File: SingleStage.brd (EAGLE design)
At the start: 47.9 x 35.5 mm, 29 parts, among them T1 2N5089

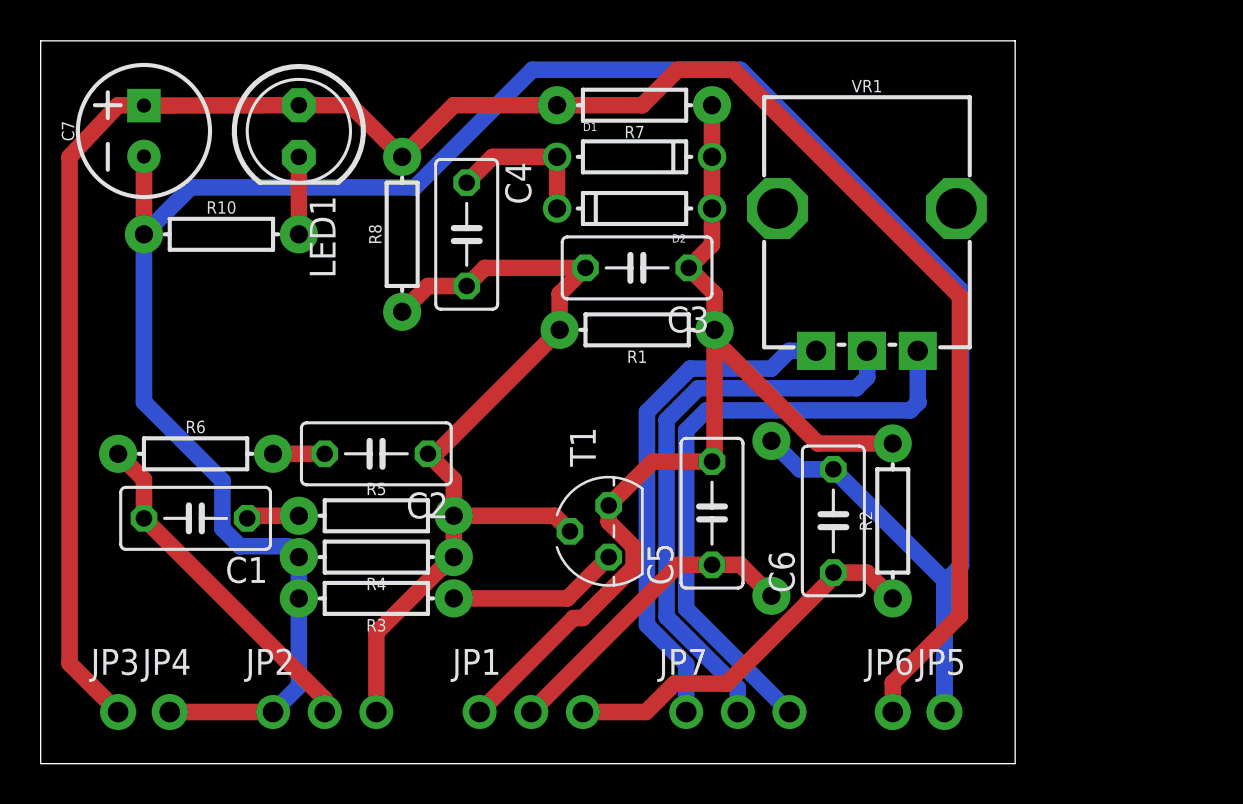
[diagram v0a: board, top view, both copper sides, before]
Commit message: Add files via upload
Layout complete ad Gerber files generated.
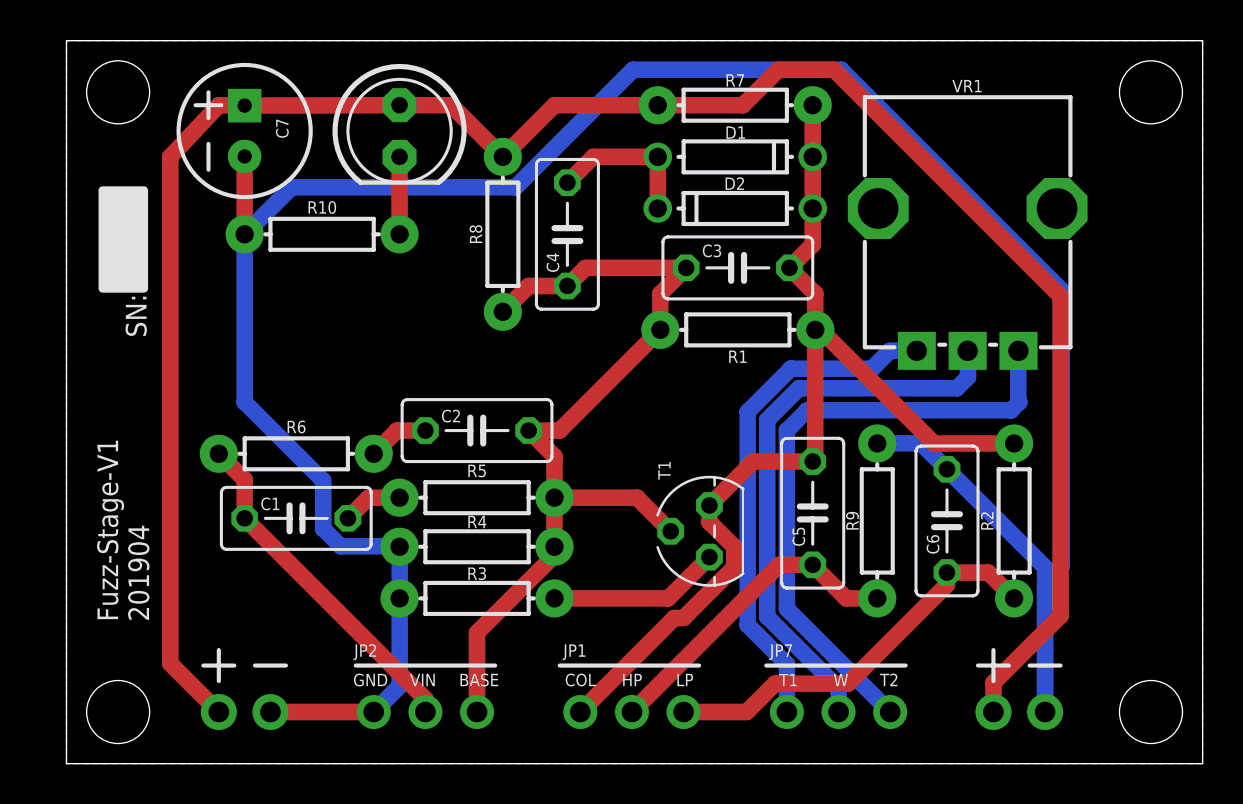
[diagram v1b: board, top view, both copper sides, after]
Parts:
- moved R2 5.97 mm to (46.6, 11.9)
- moved C6 5.59 mm to (43.3, 11.9)
- moved R9 5.21 mm to (39.9, 11.9), flipped to the top
- moved C2 5.08 mm to (20.2, 16.4)
- moved R5 5.03 mm to (20.2, 13.1)
- moved R4 4.98 mm to (20.2, 10.7)
- moved C3 4.95 mm to (33.0, 24.4)
- moved C4 4.95 mm to (24.6, 26.0)
- moved C5 4.95 mm to (36.7, 12.3)
- moved JP5 4.95 mm to (48.1, 2.54)
- moved JP6 4.95 mm to (45.6, 2.54)
- moved R1 4.95 mm to (33.0, 21.3)
- moved VR1 4.95 mm to (44.3, 27.3)
- moved C1 4.95 mm to (11.3, 12.1)
- moved R3 4.95 mm to (20.2, 8.13)
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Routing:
- net N$11: track 18.7 -> 20.0 mm
- net N$4: track 43.4 -> 44.4 mm
- added copper zone on layer 1, net +9V
- added copper zone on layer 16, net GND
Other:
- board size 47.9 x 35.5 mm -> 55.9 x 35.6 mm
- board text added: "BASE"
- board text added: "COL"
- board text added: "Fuzz-Stage-V1 201904"
- board text added: "GND"
- board text added: "HP"
- board text added: "LP"
- board text added: "SN:"
- board text added: "T1"
- board text added: "T2"
- board text added: "VIN"
- board text added: "W"
